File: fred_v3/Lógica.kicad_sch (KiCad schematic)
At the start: 5 parts, among them J10 Conn_01x03, J2 Conn_02x07_Counter_Clockwise, J3 Conn_02x07_Counter_Clockwise

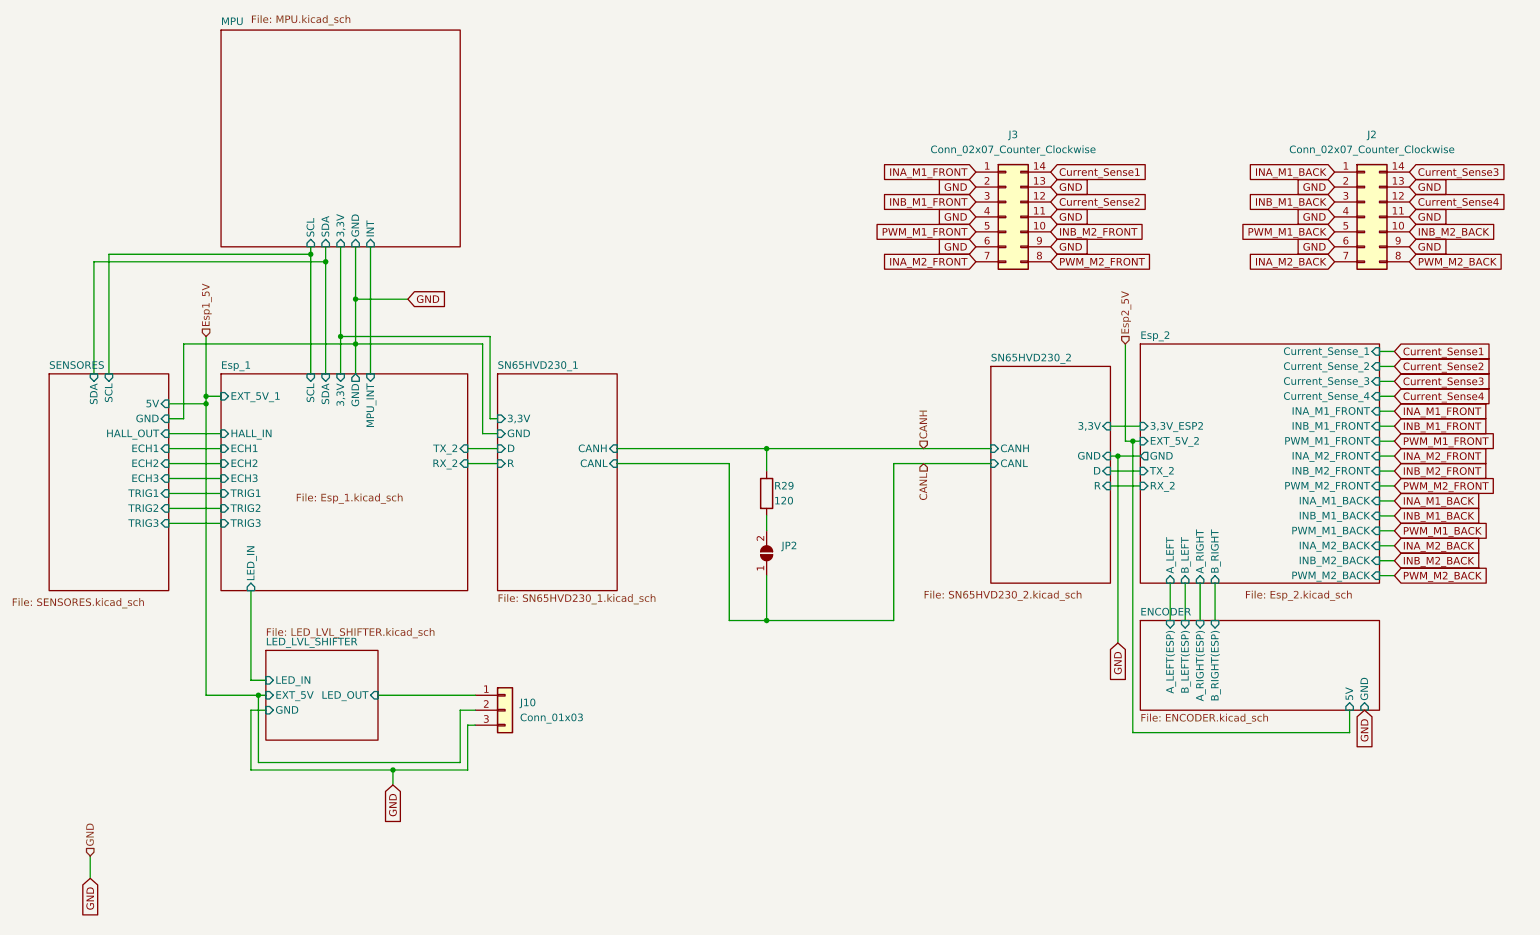
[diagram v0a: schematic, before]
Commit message: Add files via upload
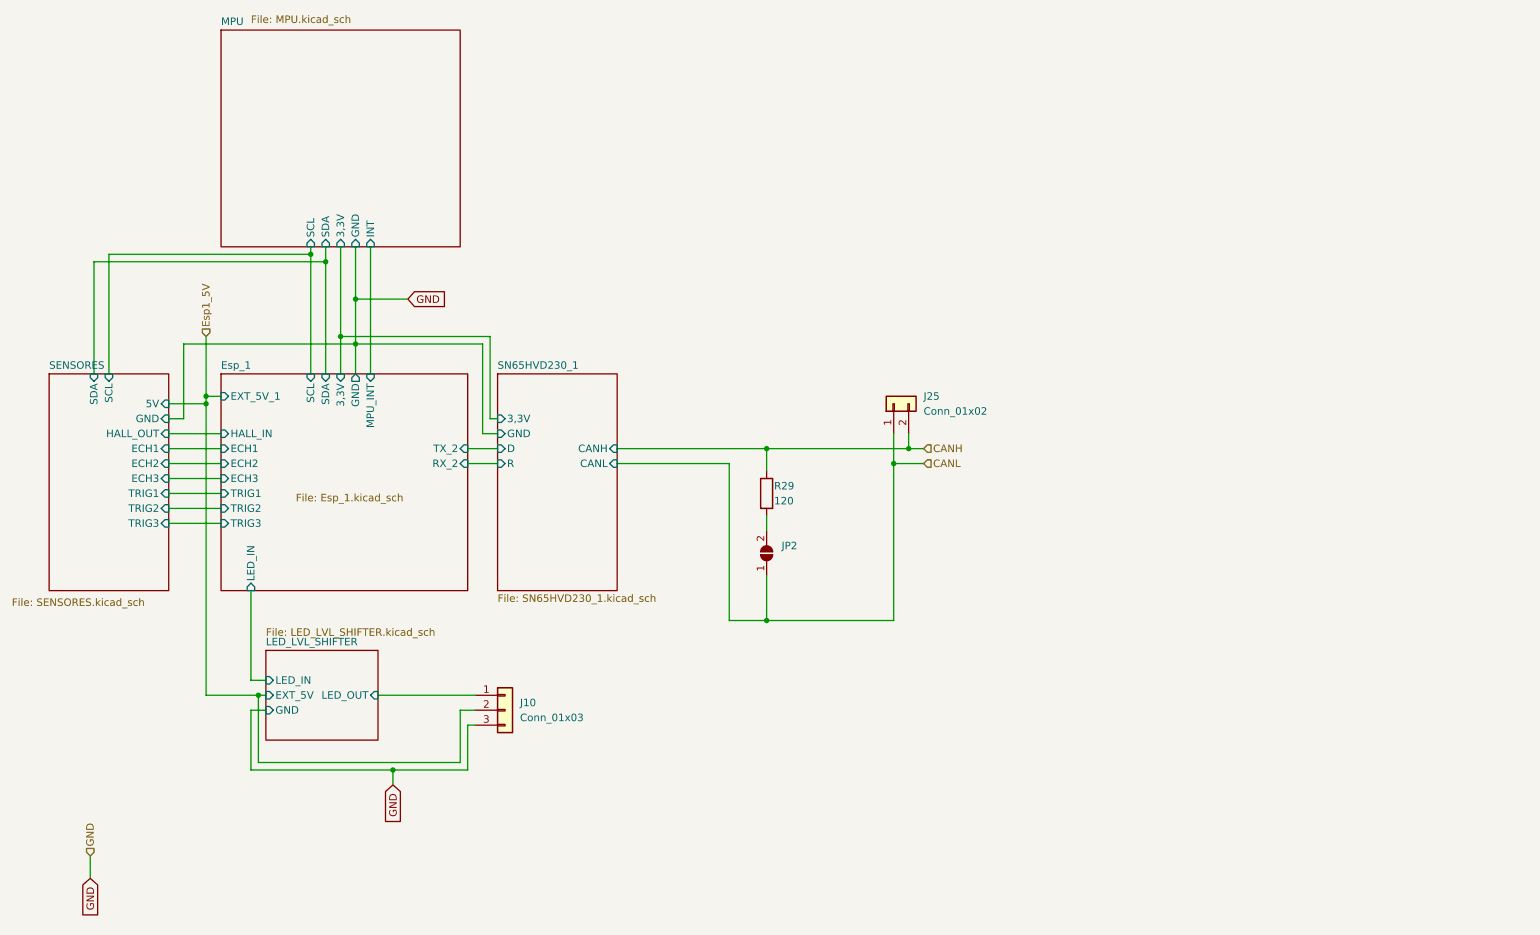
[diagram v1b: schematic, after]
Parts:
- removed J2, J3: Conn_02x07_Counter_Clockwise, Connector_IDC:IDC-Header_2x07_P2.54mm_Vertical, symbol Connector_Generic:Conn_02x07_Counter_Clockwise
- added J25: Conn_01x02, TerminalBlock_Phoenix:TerminalBlock_Phoenix_MKDS-3-2-5.08_1x02_P5.08mm_Horizontal, symbol Connector_Generic:Conn_01x02
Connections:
- net CANH: now also J25.2 (Pin_2)
- net CANL: now also J25.1 (Pin_1)
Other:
- removed sheet ENCODER
- removed sheet Esp_2
- removed sheet SN65HVD230_2
